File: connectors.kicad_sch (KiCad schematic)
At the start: 4 parts, among them J1 Conn_01x04_Pin, J2 Conn_01x04_Pin, J3 Conn_01x09_Pin, J4 Conn_02x03_Odd_Even

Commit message: Wires are connected in Schema 1
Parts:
- J1, J2: footprint (none) -> Connector_PinHeader_2.54mm:PinHeader_1x04_P2.54mm_Vertical
- J3: footprint (none) -> Connector_PinHeader_2.54mm:PinHeader_1x09_P2.54mm_Vertical
- J4: footprint (none) -> Connector_PinHeader_2.54mm:PinHeader_2x03_P2.54mm_Vertical
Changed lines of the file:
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@@
 			)
 		)
-		(property "Footprint" ""
+		(property "Footprint" "Connector_PinHeader_2.54mm:PinHeader_2x03_P2.54mm_Vertical"
 			(at 88.7372 128.0327 0)
 			(effects
@@
 			)
 		)
-		(property "Footprint" ""
+		(property "Footprint" "Connector_PinHeader_2.54mm:PinHeader_1x04_P2.54mm_Vertical"
 			(at 60.6351 89.3296 0)
 			(effects
@@
 			)
 		)
-		(property "Footprint" ""
+		(property "Footprint" "Connector_PinHeader_2.54mm:PinHeader_1x09_P2.54mm_Vertical"
 			(at 59.6081 127.6665 0)
 			(effects
@@
 			)
 		)
-		(property "Footprint" ""
+		(property "Footprint" "Connector_PinHeader_2.54mm:PinHeader_1x04_P2.54mm_Vertical"
 			(at 81.5911 89.0054 0)
 			(effects

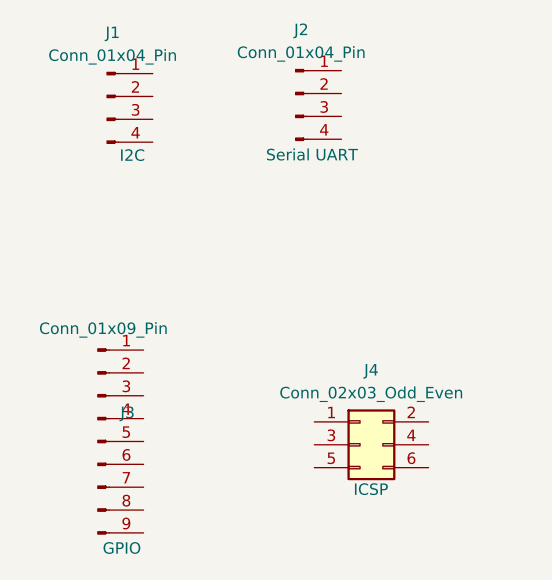
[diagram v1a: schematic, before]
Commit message: Completed wiring with electrical checker
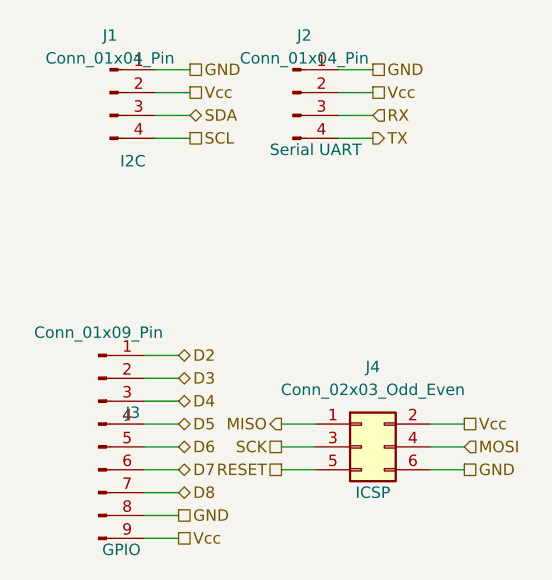
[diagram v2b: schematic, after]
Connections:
- net MISO: now reaches J4.1 (Pin_1)
- net Vcc: now reaches J4.2 (Pin_2)
- net Vcc: now also J1.2 (Pin_2), J2.2 (Pin_2), J3.9 (Pin_9)
- net SCK: now reaches J4.3 (Pin_3)
- net MOSI: now reaches J4.4 (Pin_4)
- net RESET: now reaches J4.5 (Pin_5)
- net GND: now reaches J4.6 (Pin_6)
- net GND: now also J1.1 (Pin_1), J2.1 (Pin_1), J3.8 (Pin_8)
- net SDA: now reaches J1.3 (Pin_3)
- net SCL: now reaches J1.4 (Pin_4)
- net D2: now reaches J3.1 (Pin_1)
- net D3: now reaches J3.2 (Pin_2)
- net D4: now reaches J3.3 (Pin_3)
- net D5: now reaches J3.4 (Pin_4)
- net D6: now reaches J3.5 (Pin_5)
- net D7: now reaches J3.6 (Pin_6)
- net D8: now reaches J3.7 (Pin_7)
- net RX: now reaches J2.3 (Pin_3)
- net TX: now reaches J2.4 (Pin_4)
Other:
- moved on the sheet: J1, J3
